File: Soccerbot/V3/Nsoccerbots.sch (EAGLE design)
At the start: 83 parts, among them CN2 1X4-CLEANBIG, IC2 TB6612FNG, IC4 TB6612FNG, J3 1X5, J4 1X5, Q2 AOD417, SW2 SPST_TACT-EVQQ2, U1 PCA9685, X1 NXT-SOCKET, X2 NXT-SOCKET, X3 NXT-SOCKET, X4 NXT-SOCKET

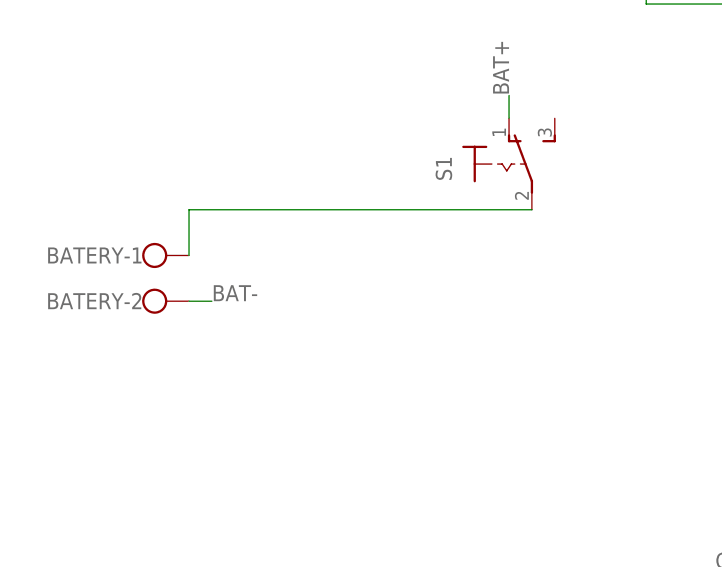
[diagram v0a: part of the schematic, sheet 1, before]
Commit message: S
S
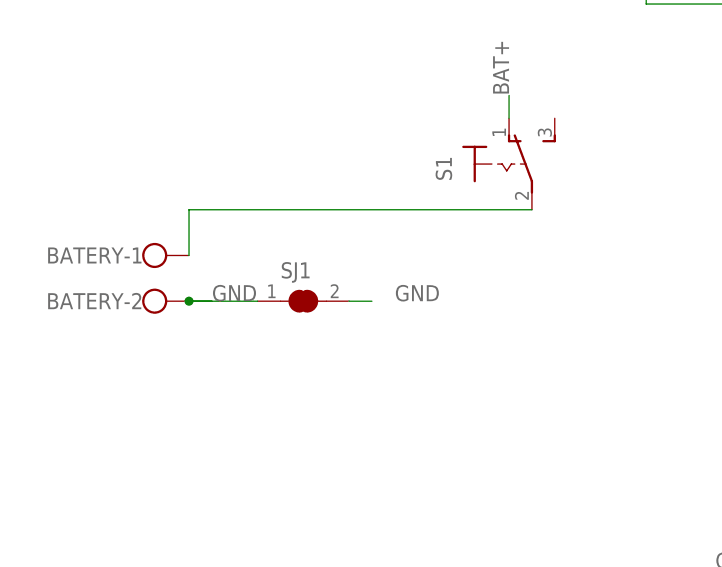
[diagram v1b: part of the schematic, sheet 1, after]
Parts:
- added SJ1: (no value), microbuilder:SOLDERJUMPER_CLOSEDPERM
- A5, A6, A7, A8, A9, CN2, D0-1, IC2, IC4, IR1, IR2, IR3, IR4, IR5, IR6, J3, J4, JP5, JP6, JP7, JP8, MPOWER1, PWR1, R1, R15, R16, R17, R19, R2, R20, R21, R22, R3, R4, R5, R6, SERPWR1, SERVO3, SERVO4, SW2, TP10, TP6, TP7, TP8, TP9, U$12, U$13, U$15: OC_NEWARK (none) -> unknown
- C11, C7, C8: MPN (none) -> 0603YC104K4Z2A; OC_NEWARK (none) -> 26M5119
- C12, C13: MPN (none) -> EEEHB1C470P; OC_NEWARK (none) -> 17AC6791
- C14: MPN (none) -> EEFCX0J101R; OC_NEWARK (none) -> 17AC6838
- C15, C16: MPN (none) -> GRM21BC80J106KE19L; OC_NEWARK (none) -> 03AC2709
- LED2: MPN (none) -> MCL-S270GC; OC_NEWARK (none) -> 14N9356
- Q2: MPN (none) -> AUIRFR540ZTRL; OC_NEWARK (none) -> 91Y4154
- R18: MF (none) -> VISHAY/DALE; MPN (none) -> CRCW12061K00FKTA; OC_NEWARK (none) -> 05F1545
- S1: MPN 5636A9 -> (none); OC_NEWARK 13M4539 -> unknown
- SJ2: MPN (none) -> 2211S-02G; OC_NEWARK (none) -> 08N6744
- U1: MPN (none) -> 6EDL04N02PRXUMA1; OC_NEWARK (none) -> 18AC0914
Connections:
- net BAT-: no longer BATERY-2.KL
- net GND: now also BATERY-2.KL, SJ1.1, SJ1.2
